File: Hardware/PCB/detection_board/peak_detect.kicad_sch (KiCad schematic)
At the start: 12 parts, among them U2 LT1807, U4 OPA365, U5 TS12A4514DBVR

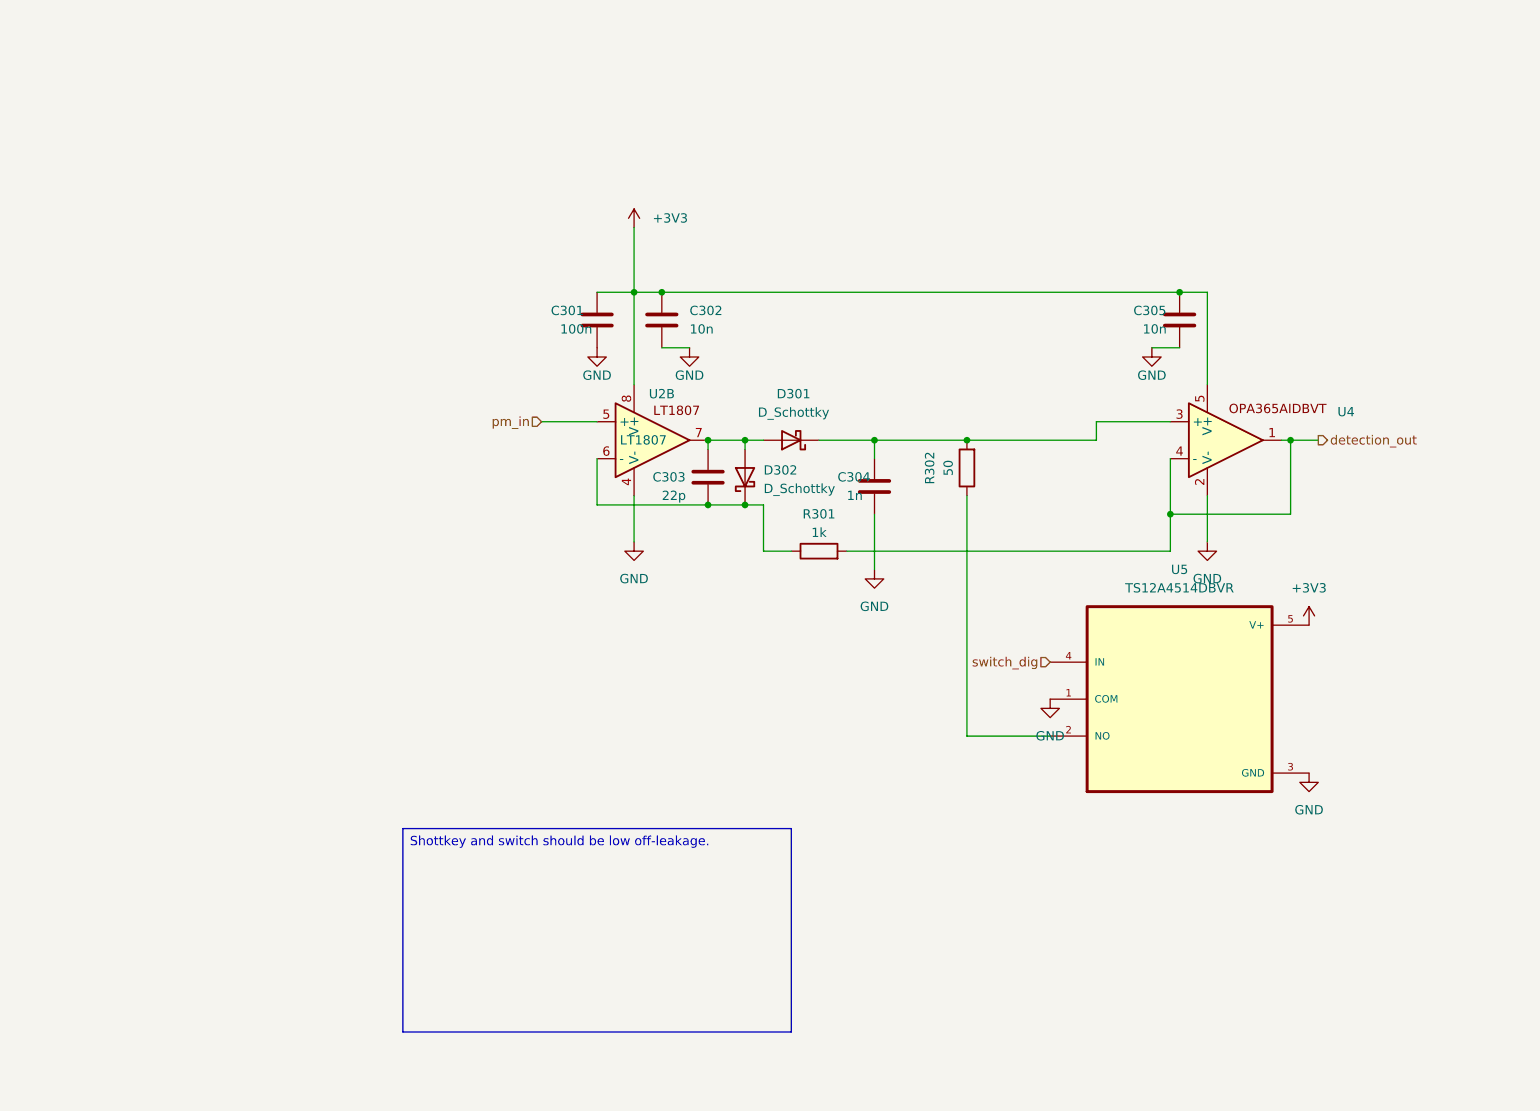
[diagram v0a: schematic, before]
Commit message: edited schematics
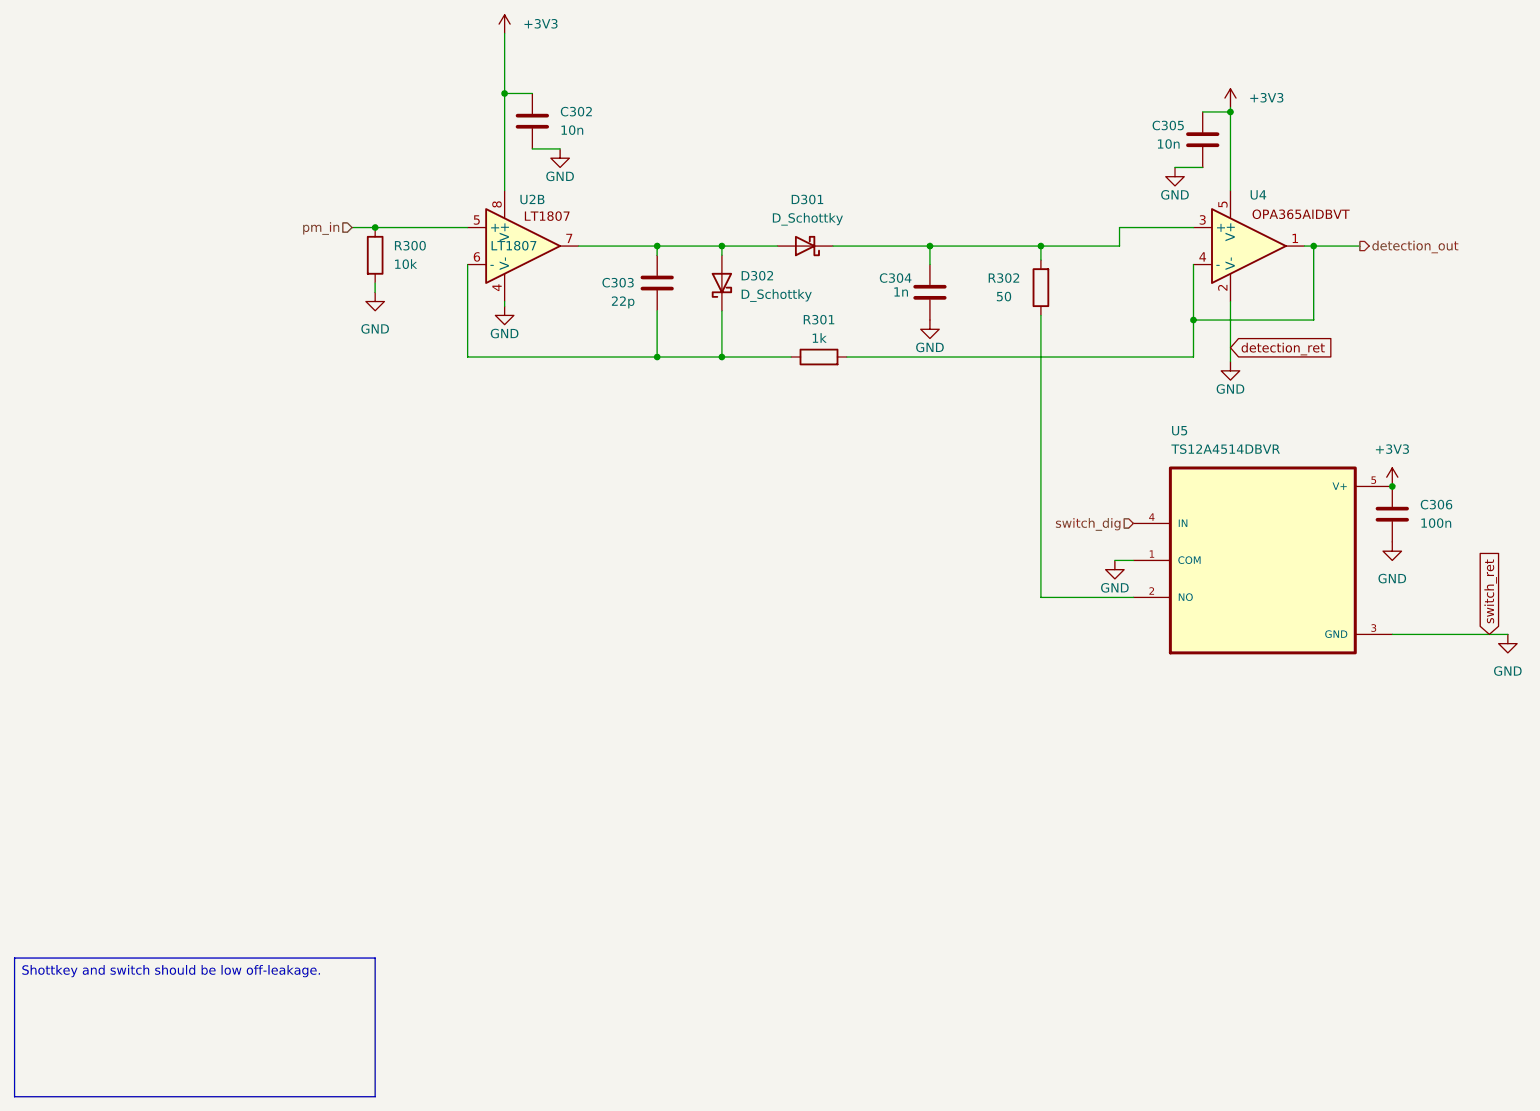
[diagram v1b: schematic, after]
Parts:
- removed C301: 100n, Capacitor_SMD:C_0805_2012Metric, symbol Device:C
- added C306: 100n, symbol Device:C
- added R300: 10k, symbol Device:R
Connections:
- net +3V3: now also C306.1
- net GND: now also C306.2, R300.2
- net pm_in: now also R300.1
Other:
- company: (none) -> UMD Nearspace Balloon Payload Program
- moved on the sheet: C302, C303, C304, C305, D301, D302, R301, R302, U2B, U4, U5
